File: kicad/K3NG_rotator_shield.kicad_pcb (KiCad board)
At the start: 2 copper layers, 68.6 x 53.3 mm, 8 parts, among them P1 Power, P2 Analog, P3 Digital, P4 Digital, P5 CONN_01X01, P6 CONN_01X01, P7 CONN_01X01, P8 CONN_01X01

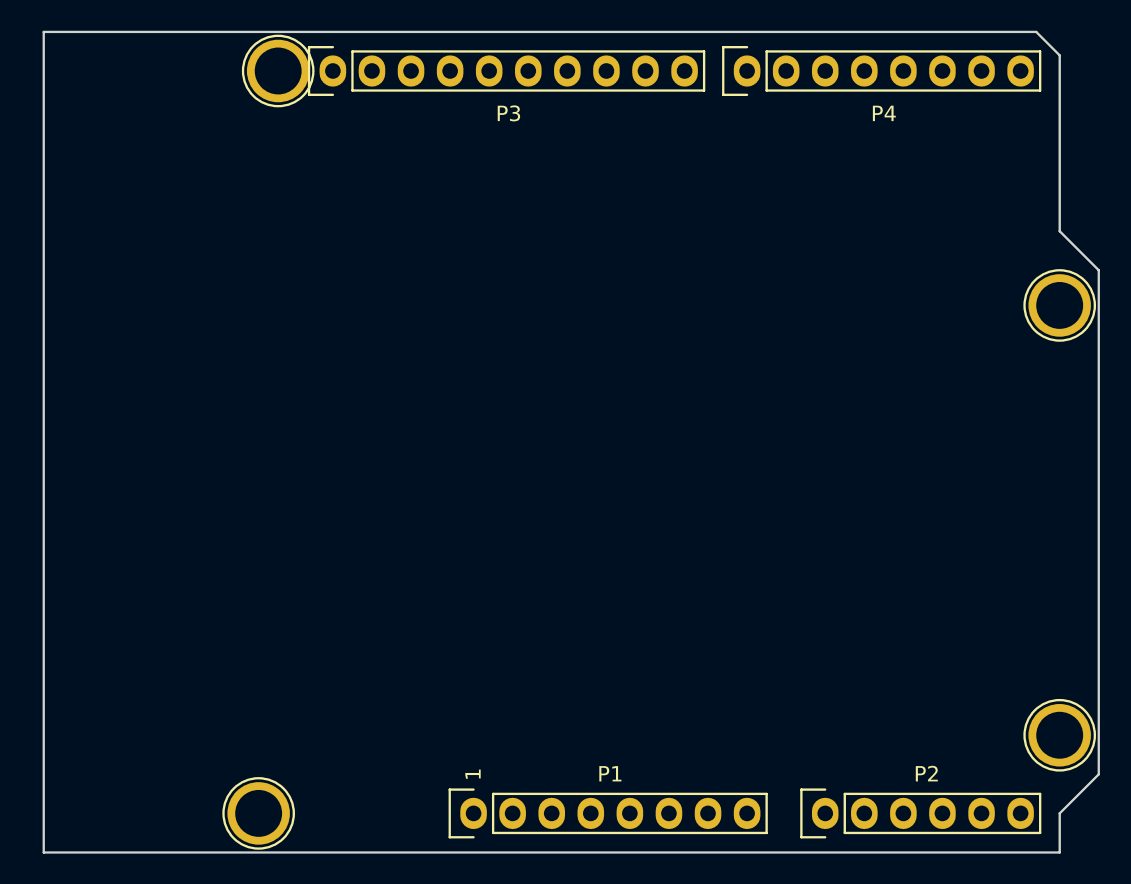
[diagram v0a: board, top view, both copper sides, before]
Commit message: Ready for final proofread
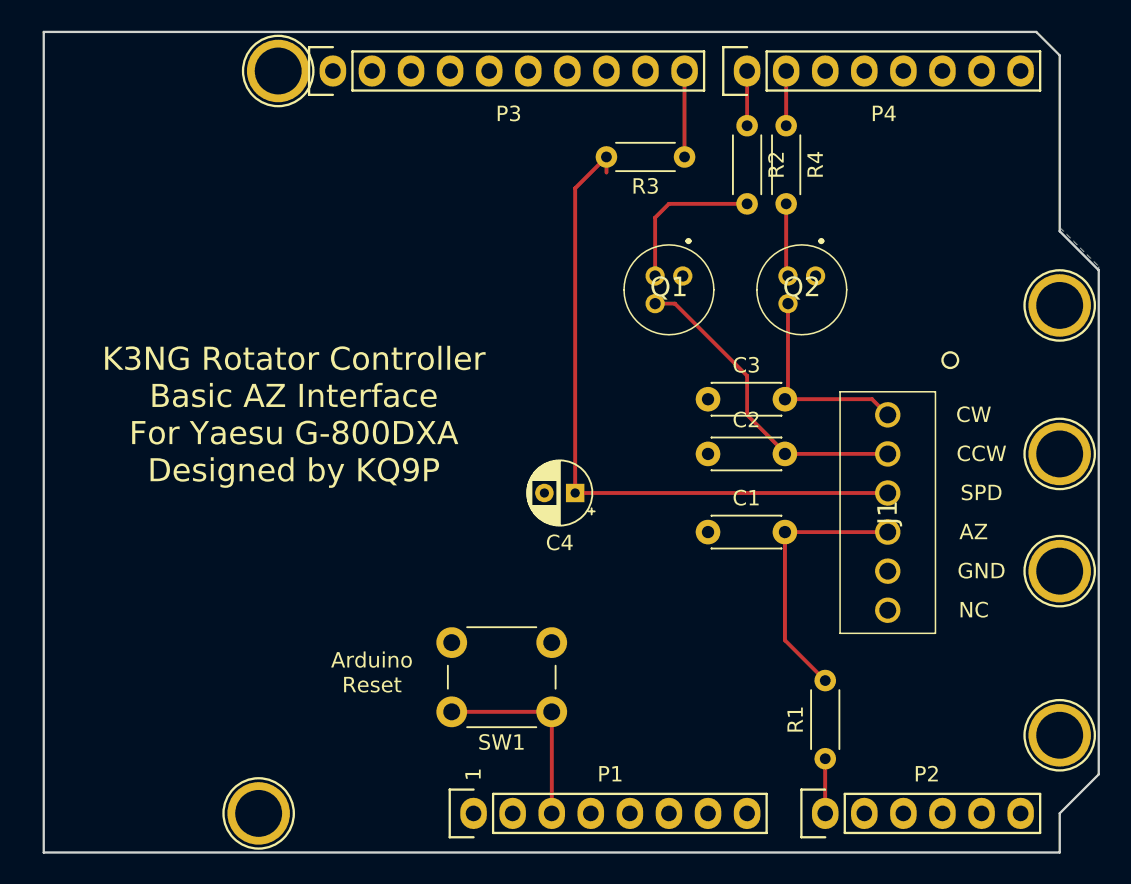
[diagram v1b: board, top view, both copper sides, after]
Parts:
- added C1: .01u, Capacitor_THT:C_Disc_D4.3mm_W1.9mm_P5.00mm, F.Cu at (154.2, 105.5)
- added C2: .01u, Capacitor_THT:C_Disc_D4.3mm_W1.9mm_P5.00mm, F.Cu at (154.2, 100.5)
- added C3: .01u, Capacitor_THT:C_Disc_D4.3mm_W1.9mm_P5.00mm, F.Cu at (154.2, 96.9)
- added C4: 10u, Capacitor_THT:CP_Radial_D4.0mm_P2.00mm, F.Cu at (145.5, 103.0)
- added J1: Screw_Terminal_01x06, SamacSys_Parts:1725698, F.Cu at (165.9, 97.9)
- added P8: CONN_01X01, Socket_Arduino_Uno:Arduino_1pin, F.Cu at (177.0, 108.1)
- added P8: CONN_01X01, Socket_Arduino_Uno:Arduino_1pin, F.Cu at (177.0, 100.5)
- added Q1: 2N2222Ae3, SamacSys_Parts:JANTX2N2222A, F.Cu at (151.6, 89.8)
- added Q2: 2N2222Ae3, SamacSys_Parts:JANTX2N2222A, F.Cu at (160.3, 89.8)
- added R1: 1k, Resistor_THT:R_Axial_DIN0204_L3.6mm_D1.6mm_P5.08mm_Horizontal, F.Cu at (161.8, 120.3)
- added R2: 1k, Resistor_THT:R_Axial_DIN0204_L3.6mm_D1.6mm_P5.08mm_Horizontal, F.Cu at (156.7, 79.1)
- added R3: 4k7, Resistor_THT:R_Axial_DIN0204_L3.6mm_D1.6mm_P5.08mm_Horizontal, F.Cu at (152.7, 81.2)
- added R4: 1k, Resistor_THT:R_Axial_DIN0204_L3.6mm_D1.6mm_P5.08mm_Horizontal, F.Cu at (159.3, 79.1)
- added SW1: SW_Push_Dual, Button_Switch_THT:SW_PUSH_6mm_H4.3mm, F.Cu at (144.0, 117.2)
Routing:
- net /SPDctlr: track 0.00 -> 44.0 mm
- net /CCWctlr: track 0.00 -> 20.7 mm
- net /AZctlr: track 0.00 -> 17.4 mm
- net /CWctlr: track 0.00 -> 13.4 mm
- net /Reset: track 0.00 -> 13.1 mm
- net Net-(Q1-Pad2): track 0.00 -> 10.1 mm
- net /8: track 0.00 -> 5.59 mm
- net Net-(Q2-Pad2): track 0.00 -> 4.74 mm
- net /A0: track 0.00 -> 3.56 mm
- net /7: track 0.00 -> 3.56 mm
- net /6(**): track 0.00 -> 3.56 mm
- added copper zone on B.Cu, net GND
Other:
- board text added: "AZ"
- board text added: "Arduino Reset"
- board text added: "CCW"
- board text added: "CW"
- board text added: "GND"
- board text added: "K3NG Rotator Controller Basic AZ Interface For Yaesu G-800DXA Designed by KQ9P"
- board text added: "NC"
- board text added: "SPD"
